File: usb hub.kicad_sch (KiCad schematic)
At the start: 1 part, among them J1 TYPE-C-31-M-12

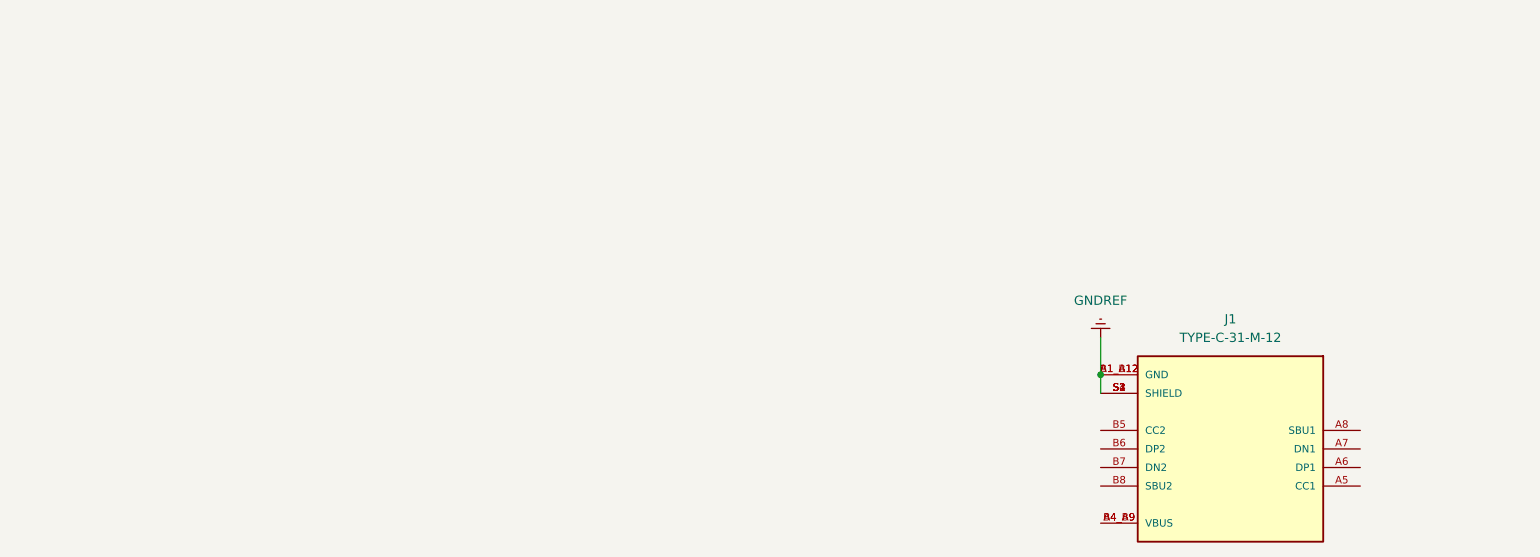
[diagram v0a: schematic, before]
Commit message: more updates!
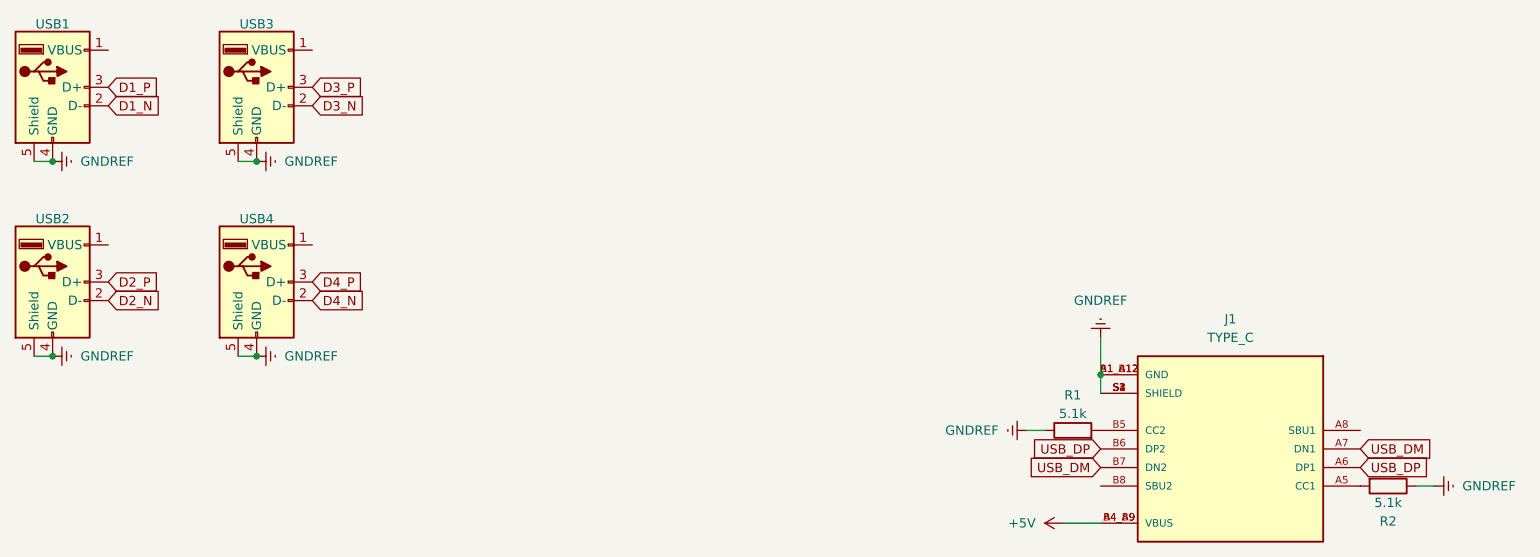
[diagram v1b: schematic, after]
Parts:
- added R1, R2: 5.1k, RMCF0805JT5K10:RESC2012X65N, symbol Device:R
- added USB1, USB2, USB3, USB4: USB_A, symbol Connector:USB_A
- J1: value TYPE-C-31-M-12 -> TYPE_C
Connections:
- net GNDREF: now also R1.1, R2.1, USB1.4 (GND), USB1.5 (Shield), USB2.4 (GND), USB2.5 (Shield), USB3.4 (GND), USB3.5 (Shield), USB4.4 (GND), USB4.5 (Shield)
- net +5V: now reaches J1.A4_B9 (VBUS), J1.B4_A9 (VBUS)
- net at J1.A5 (CC1): now also R2.2
- net USB_DP: now reaches J1.A6 (DP1)
- net USB_DP: now also J1.B6 (DP2)
- net USB_DM: now reaches J1.A7 (DN1)
- net USB_DM: now also J1.B7 (DN2)
- net at J1.B5 (CC2): now also R1.2
- new net D1_N: USB1.2 (D-)
- new net D1_P: USB1.3 (D+)
- new net D2_N: USB2.2 (D-)
- new net D2_P: USB2.3 (D+)
- new net D3_N: USB3.2 (D-)
- new net D3_P: USB3.3 (D+)
- new net D4_N: USB4.2 (D-)
- new net D4_P: USB4.3 (D+)
